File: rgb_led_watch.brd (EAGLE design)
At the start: 50.3 x 66.1 mm, 38 parts, among them IC4 74V1T126CTR, U1 AT42QT1010SOT23

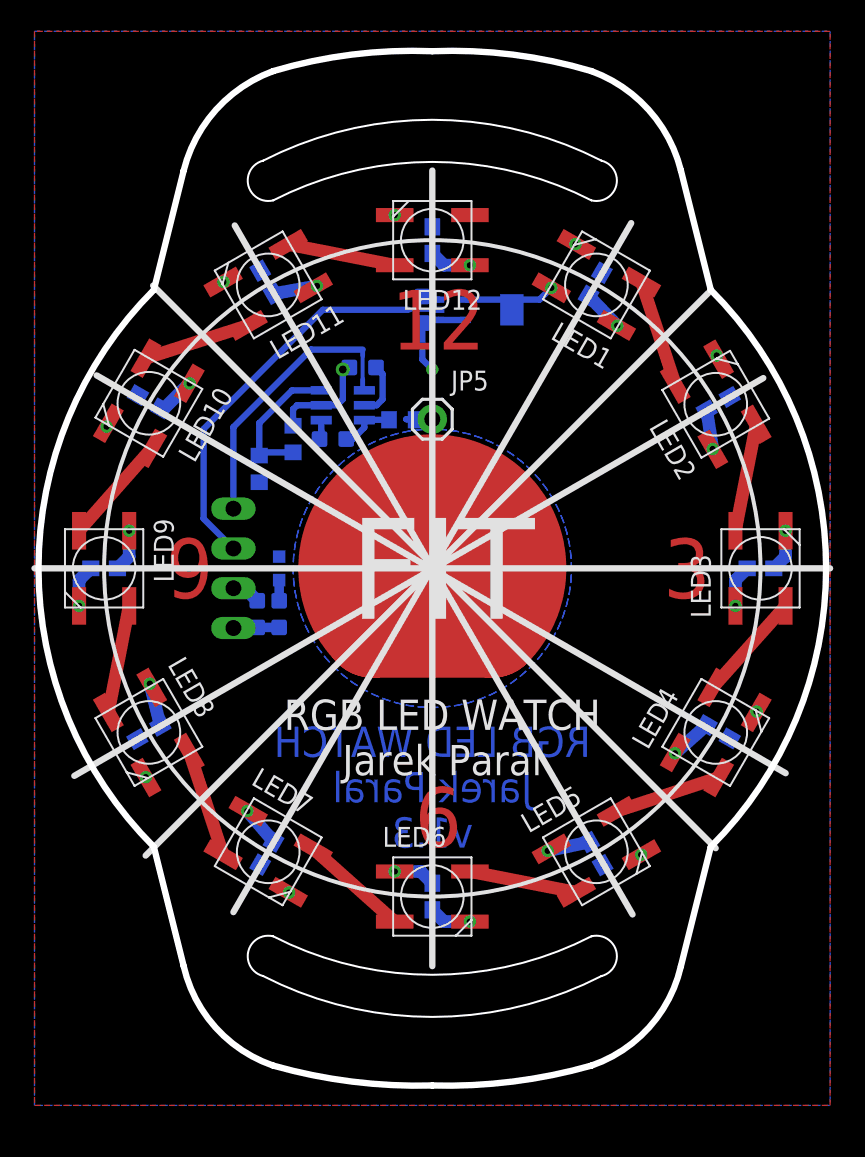
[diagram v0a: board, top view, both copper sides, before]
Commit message: hodinky
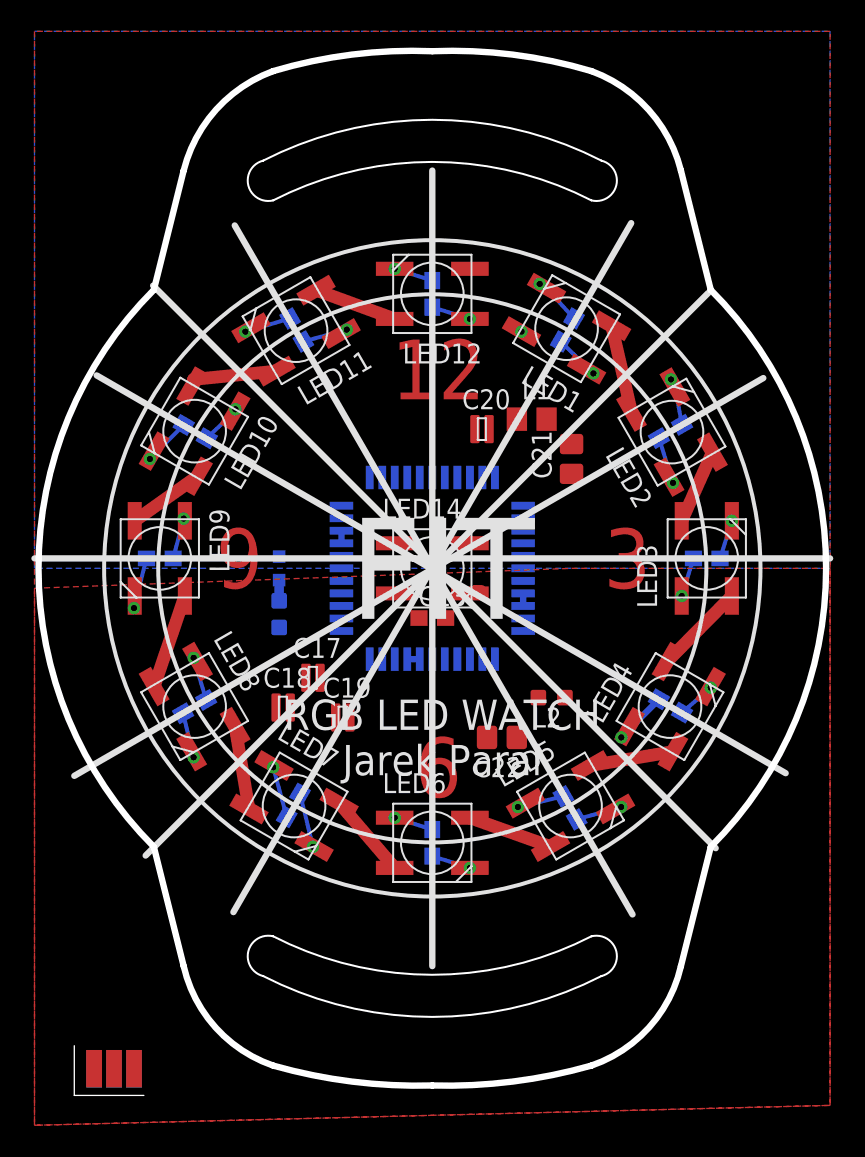
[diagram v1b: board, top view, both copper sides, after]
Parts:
- removed C14, C16: 100n/6,3V, rcl_upravena:C0603
- removed C15: 10n, rcl_upravena:C0603
- removed IC4: 74V1T126CTR, 74xx-little-de:SC70-5
- removed JP1: (no value), pinhead:1X04/90
- removed JP5: M01PTH, SparkFun-Connectors:1X01
- removed JP9: M01SMD-4.5X1.5, SparkFun-Connectors:PAD-1.5X4.5
- removed R1: 10k, rcl:R0603
- removed R2_LOW, R3_FAST: 0, rcl:R0603
- removed U1: AT42QT1010SOT23, SparkFun-DigitalIC:SOT23-6
- added C17, C18, C19, C20: 100nF, rcl_upravena:C0306
- added C21, C22: 10nF, rcl_upravena:C0805
- added L1: 10uH, rcl_upravena:R0805
- added L2: FB, rcl_upravena:R0603
- added LED14: WS2812B, rgb_led:WS2812B
- added U$1: CON_PROG-6CORN, con_prog:SMD-6-CORNER
- added U$2: ATXMEGA128A4U_AU, xmega:TQFP44
- C13: value 4u7 -> 100n; device rcl_upravena:C0603 -> resistor:C0603
- moved C13 11.2 mm to (50.8, 47.6), flipped to the top, turned to 0 degrees
- moved C9 3.61 mm to (33.4, 51.4)
- moved LED9 3.61 mm to (33.4, 51.4)
- moved C11 3.59 mm to (42.1, 66.0)
- moved C2 3.53 mm to (66.0, 59.5)
- moved C3 3.49 mm to (68.3, 51.4)
- moved LED3 3.49 mm to (68.3, 51.4)
- moved C10 3.49 mm to (35.7, 59.5)
- moved C7 3.49 mm to (41.9, 35.7), turned to 300 degrees
- moved C4 3.47 mm to (66.0, 42.0)
- moved C12 3.43 mm to (50.8, 68.3)
- moved C6 3.43 mm to (50.8, 33.3)
- moved LED12 3.43 mm to (50.8, 68.3)
- moved LED6 3.43 mm to (50.8, 33.3)
- moved LED10 3.42 mm to (35.6, 59.6)
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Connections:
- removed net PAD: JP5.1, R1.2
- removed net SIG_IN: IC4.2, JP1.2
- removed net SNS: C15.2, U1.4
- removed net SNSK: C15.1, R1.1, U1.3
- removed net SWITCH: JP1.1, U1.1
- removed net SYNC_MODE: R2_LOW.2, R3_FAST.1, U1.6
- new net +3V3: L1.1, U$1.P$2
- new net N$1: C17.2, C18.2, C19.2, C21.2, L1.2, L2.1
- new net N$11: C20.1, C22.1, L2.2, U$2.39
- new net N$12: U$1.P$1, U$2.34
- new net N$13: U$1.P$3, U$2.33
- new net N$14: U$1.P$4, U$2.32
- new net N$15: U$1.P$5, U$2.35
- new net N$16: LED12.DOUT, LED14.DIN
- net +5V: now also C13.2, LED14.VDD; no longer C13.1, C14.2, C16.1, IC4.1, IC4.5, JP1.4, R3_FAST.2, U1.5
- net GND: now also C13.1, C17.1, C18.1, C19.1, C20.2, C21.1, C22.2, LED14.VSS, U$1.P$6, U$2.18, U$2.19, U$2.30, U$2.31, U$2.38, U$2.8, U$2.9; no longer C13.2, C14.1, C16.2, IC4.3, JP1.3, R2_LOW.1, U1.2
- net SIG_OUT: now also U$2.23; no longer IC4.4, JP9.P$1
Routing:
- net PAD: track 44.9 -> 0.00 mm
- net SIG_IN: track 26.6 -> 0.00 mm
- net GND: track 16.0 -> 42.1 mm
- net SWITCH: track 19.1 -> 0.00 mm
- net +5V: track 52.4 -> 37.6 mm, vias 14 -> 12
- net SYNC_MODE: track 9.14 -> 0.00 mm
- net SIG_OUT: track 6.44 -> 0.00 mm
- net SNSK: track 3.52 -> 0.00 mm
- net N$5: track 6.93 -> 4.81 mm
- net LED2: track 7.02 -> 4.92 mm
- net N$10: track 6.93 -> 5.35 mm
- net N$7: track 6.87 -> 5.33 mm
- net N$4: track 6.87 -> 5.33 mm
- net LED1: track 6.97 -> 5.45 mm
- net N$6: track 6.93 -> 5.47 mm
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- added copper zone on layer 1, net GND
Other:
- board text removed: "AT42QT1010"
- board text removed: "Breakout"
- board text removed: "RGB LED WATCH Jarek Paral v1.3"
